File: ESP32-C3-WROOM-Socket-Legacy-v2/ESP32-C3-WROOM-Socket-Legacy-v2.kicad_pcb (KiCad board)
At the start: 2 copper layers, 35.6 x 35.6 mm, 6 parts, among them SW1 SW_Push, U2 ESP32-C3-WROOM-02-N4

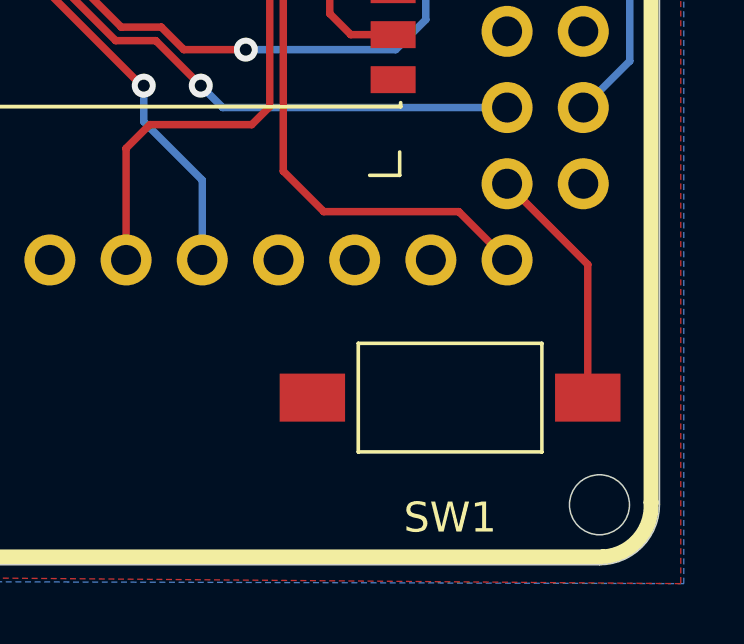
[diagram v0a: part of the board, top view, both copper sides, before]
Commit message: .
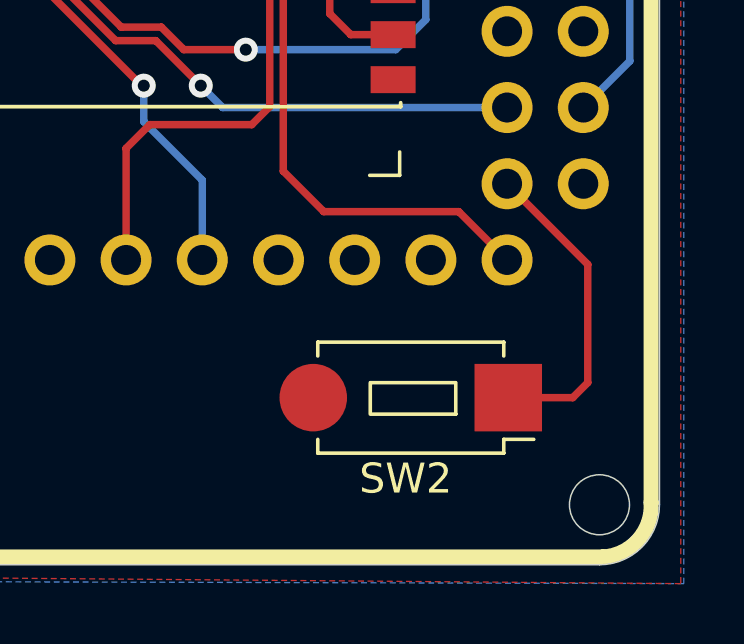
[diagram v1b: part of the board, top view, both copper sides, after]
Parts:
- removed SW1: SW_Push, Alexander Footprint Library:SW_SPST_6x3
- added SW2: SW_Push_SMD_6x3.5, Alexander Footprint Library:SW_PUSH_6x3.5mm, F.Cu at (220.7, 106.2)
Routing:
- net /GPIO0: track 28.6 -> 30.9 mm
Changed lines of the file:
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@@
 		)
 	)
-	(footprint "Alexander Footprint Library:SW_SPST_6x3"
-		(layer "F.Cu")
-		(at 218.71 106.2 180)
-		(tags "SPST button tactile switch")
-		(property "Reference" "SW1"
-			(at 0 -4 0)
+	(footprint "Alexander Footprint Library:SW_PUSH_6x3.5mm"
+		(layer "F.Cu")
+		(at 220.65 106.2 180)
+		(descr "tactile push button, 6x3.5mm, https://www.apem.com/idec-apem/en_US/PCB-switches/Tactile-Switches/MJTP-6mm-through-hole/c/MJTP_6mm_through%20hole?page=1")
+		(tags "PHAP3362 6mm tact sw THT")
+		(property "Reference" "SW2"
+			(at 3.42 -2.7 0)
 			(layer "F.SilkS")
 			(effects
@@
 			)
 		)
-		(property "Value" "SW_Push"
-			(at 0 3 0)
+		(property "Value" "SW_Push_SMD_6x3.5"
+			(at 4.4 3.7 0)
 			(layer "F.Fab")
 			(effects
@@
 			)
 		)
-		(property "Footprint" "Alexander Footprint Library:SW_SPST_6x3"
+		(property "Footprint" "Alexander Footprint Library:SW_PUSH_6x3.5mm"
 			(at 0 0 180)
 			(unlocked yes)
@@
 			)
 		)
-		(property "Description" "Push button switch, generic, two pins"
+		(property "Description" ""
 			(at 0 0 180)
 			(unlocked yes)
@@
 		(sheetname "Root")
 		(sheetfile "ESP32-C3-WROOM-Socket-Legacy-v2.kicad_sch")
-		(attr smd)
-		(fp_line
-			(start 3.06 1.81)
-			(end -3.06 1.81)
+		(attr through_hole)
+		(fp_line
+			(start 6.35 1.39)
+			(end 6.35 1.85)
 			(stroke
 				(width 0.12)
@@
 		)
 		(fp_line
-			(start 3.06 -1.81)
-			(end 3.06 1.81)
+			(start 6.35 -1.85)
+			(end 6.35 -1.39)
 			(stroke
 				(width 0.12)
@@
 		)
 		(fp_line
-			(start -3.06 1.81)
-			(end -3.06 -1.81)
+			(start 6.35 -1.85)
+			(end 0.15 -1.85)
 			(stroke
 				(width 0.12)
@@
 		)
 		(fp_line
-			(start -3.06 -1.81)
-			(end 3.06 -1.81)
+			(start 0.15 1.85)
+			(end 6.35 1.85)
 			(stroke
 				(width 0.12)
@@
 		)
 		(fp_line
-			(start 5.95 -2)
-			(end 5.95 2)
-			(stroke
-				(width 0.05)
-				(type solid)
-			)
-			(layer "F.CrtYd")
-		)
-		(fp_line
-			(start -5.95 2)
-			(end 5.95 2)
-			(stroke
-				(width 0.05)
-				(type solid)
-			)
-			(layer "F.CrtYd")
-		)
-		(fp_line
-			(start -5.95 -2)
-			(end 5.95 -2)
-			(stroke
-				(width 0.05)
-				(type solid)
-			)
-			(layer "F.CrtYd")
-		)
-		(fp_line
-			(start -5.95 -2)
-			(end -5.95 2)
-			(stroke
-				(width 0.05)
-				(type solid)
-			)
-			(layer "F.CrtYd")
-		)
-		(fp_line
-			(start 3 -1.75)
-			(end 3 1.75)
-			(stroke
-				(width 0.1)
-				(type solid)
-			)
-			(layer "F.Fab")
-		)
-		(fp_line
-			(start 1.75 1)
-			(end -1.75 1)
-			(stroke
-				(width 0.1)
-				(type solid)
-			)
-			(layer "F.Fab")
-		)
-		(fp_line
-			(start 1.75 -1)
-			(end 1.75 1)
-			(stroke
-				(width 0.1)
-				(type solid)
-			)
-			(layer "F.Fab")
-		)
-		(fp_line
-			(start 1.5 -0.8)
-			(end 1.5 0.8)
-			(stroke
-				(width 0.1)
-				(type solid)
-			)
-			(layer "F.Fab")
-		)
-		(fp_line
-			(start -1.5 0.8)
-			(end 1.5 0.8)
-			(stroke
-				(width 0.1)
-				(type solid)
-			)
-			(layer "F.Fab")
-		)
-		(fp_line
-			(start -1.5 -0.8)
-			(end 1.5 -0.8)
-			(stroke
-				(width 0.1)
-				(type solid)
-			)
-			(layer "F.Fab")
-		)
-		(fp_line
-			(start -1.5 -0.8)
-			(end -1.5 0.8)
-			(stroke
-				(width 0.1)
-				(type solid)
-			)
-			(layer "F.Fab")
-		)
-		(fp_line
-			(start -1.75 1)
-			(end -1.75 -1)
-			(stroke
-				(width 0.1)
-				(type solid)
-			)
-			(layer "F.Fab")
-		)
-		(fp_line
-			(start -1.75 -1)
-			(end 1.75 -1)
-			(stroke
-				(width 0.1)
-				(type solid)
-			)
-			(layer "F.Fab")
-		)
-		(fp_line
-			(start -3 1.75)
-			(end 3 1.75)
-			(stroke
-				(width 0.1)
-				(type solid)
-			)
-			(layer "F.Fab")
-		)
-		(fp_line
-			(start -3 -1.75)
-			(end 3 -1.75)
-			(stroke
-				(width 0.1)
-				(type solid)
-			)
-			(layer "F.Fab")
-		)
-		(fp_line
-			(start -3 -1.75)
-			(end -3 1.75)
+			(start 0.15 1.39)
+			(end 0.15 1.85)
+			(stroke
+				(width 0.12)
+				(type solid)
+			)
+			(layer "F.SilkS")
+		)
+		(fp_line
+			(start 0.15 -1.39)
+			(end -0.85 -1.39)
+			(stroke
+				(width 0.12)
+				(type default)
+			)
+			(layer "F.SilkS")
+		)
+		(fp_line
+			(start 0.15 -1.85)
+			(end 0.15 -1.39)
+			(stroke
+				(width 0.12)
+				(type default)
+			)
+			(layer "F.SilkS")
+		)
+		(fp_rect
+			(start 1.75 -0.55)
+			(end 4.6 0.5)
+			(stroke
+				(width 0.12)
+				(type default)
+			)
+			(fill none)
+			(layer "F.SilkS")
+		)
+		(fp_line
+			(start 6.5 2)
+			(end 0 2)
+			(stroke
+				(width 0.05)
+				(type solid)
+			)
+			(layer "F.CrtYd")
+		)
+		(fp_line
+			(start 6.5 1.38)
+			(end 6.5 2)
+			(stroke
+				(width 0.05)
+				(type default)
+			)
+			(layer "F.CrtYd")
+		)
+		(fp_line
+			(start 6.5 -2)
+			(end 6.5 -1.38)
+			(stroke
+				(width 0.05)
+				(type default)
+			)
+			(layer "F.CrtYd")
+		)
+		(fp_line
+			(start 0 1.38)
+			(end 0 2)
+			(stroke
+				(width 0.05)
+				(type default)
+			)
+			(layer "F.CrtYd")
+		)
+		(fp_line
+			(start 0 -2)
+			(end 6.5 -2)
+			(stroke
+				(width 0.05)
+				(type solid)
+			)
+			(layer "F.CrtYd")
+		)
+		(fp_line
+			(start 0 -2)
+			(end 0 -1.38)
+			(stroke
+				(width 0.05)
+				(type default)
+			)
+			(layer "F.CrtYd")
+		)
+		(fp_line
+			(start -1.38 1.38)
+			(end 0 1.38)
+			(stroke
+				(width 0.05)
+				(type default)
+			)
+			(layer "F.CrtYd")
+		)
+		(fp_line
+			(start -1.38 1.38)
+			(end -1.38 -1.38)
+			(stroke
+				(width 0.05)
+				(type solid)
+			)
+			(layer "F.CrtYd")
+		)
+		(fp_line
+			(start -1.38 -1.38)
+			(end 0 -1.38)
+			(stroke
+				(width 0.05)
+				(type default)
+			)
+			(layer "F.CrtYd")
+		)
+		(fp_arc
+			(start 6.5 -1.38)
+			(mid 7.88 0)
+			(end 6.5 1.38)
+			(stroke
+				(width 0.05)
+				(type default)
+			)
+			(layer "F.CrtYd")
+		)
+		(fp_line
+			(start 6.25 1.75)
+			(end 0.25 1.75)
+			(stroke
+				(width 0.1)
+				(type solid)
+			)
+			(layer "F.Fab")
+		)
+		(fp_line
+			(start 6.25 -1.75)
+			(end 6.25 1.75)
+			(stroke
+				(width 0.1)
+				(type solid)
+			)
+			(layer "F.Fab")
+		)
+		(fp_line
+			(start 0.65 -1.75)
+			(end 6.25 -1.75)
+			(stroke
+				(width 0.1)
+				(type solid)
+			)
+			(layer "F.Fab")
+		)
+		(fp_line
+			(start 0.65 -1.75)
+			(end 0.25 -1.35)
+			(stroke
+				(width 0.1)
+				(type default)
+			)
+			(layer "F.Fab")
+		)
+		(fp_line
+			(start 0.25 1.75)
+			(end 0.25 -1.35)
 			(stroke
 				(width 0.1)
@@
 		)
 		(fp_text user "${REFERENCE}"
-			(at 0 -2.6 0)
+			(at 3 0 0)
 			(layer "F.Fab")
 			(effects
@@
 		)
 		(pad "1" smd rect
-			(at -4.59 0 180)
-			(size 2.18 1.6)
+			(at 0 0 270)
+			(size 2.25 2.25)
 			(layers "F.Cu" "F.Paste" "F.Mask")
 			(net 4 "/GPIO0")
@@
 			(pintype "passive")
 		)
-		(pad "2" smd rect
-			(at 4.59 0 180)
-			(size 2.18 1.6)
+		(pad "2" smd oval
+			(at 6.5 0 270)
+			(size 2.25 2.25)
 			(layers "F.Cu" "F.Paste" "F.Mask")
 			(net 1 "GND")
@@
 			(pintype "passive")
 		)
-		(model "${KICAD8_3DMODEL_DIR}/Button_Switch_SMD.3dshapes/SW_SPST_FSMSM.wrl"
+		(model "${KICAD8_3DMODEL_DIR}/Button_Switch_THT.3dshapes/SW_PUSH_1P1T_6x3.5mm_H4.3_APEM_MJTP1243.wrl"
 			(offset
 				(xyz 0 0 0)
@@
 	(segment
 		(start 223.3 101.76)
-		(end 220.61 99.07)
+		(end 223.3 105.7)
+		(width 0.25)
+		(layer "F.Cu")
+		(net 4)
+	)
+	(segment
+		(start 223.3 105.7)
+		(end 222.8 106.2)
+		(width 0.25)
+		(layer "F.Cu")
+		(net 4)
+	)
+	(segment
+		(start 222.8 106.2)
+		(end 220.65 106.2)
 		(width 0.25)
 		(layer "F.Cu")
@@
 	)
 	(segment
+		(start 220.61 99.07)
+		(end 223.3 101.76)
+		(width 0.25)
+		(layer "F.Cu")
+		(net 4)
+	)
+	(segment
 		(start 217.6 83.6)
 		(end 216.8125 83.6)
 		(width 0.25)
 		(layer "F.Cu")
-		(net 4)
-	)
-	(segment
-		(start 223.3 106.2)
-		(end 223.3 101.76)
-		(width 0.25)
-		(layer "F.Cu")
